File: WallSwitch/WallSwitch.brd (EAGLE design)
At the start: 72 x 54 mm, 37 parts, among them IC1 WS2811, IC2 AT42QT1010-TSHR, IC3 LNK306DG, IC4 WS2811, IC5 AT42QT1010-TSHR, IC6 AP2112K-3.3TRG1, J1 AC Line, J2 Interface

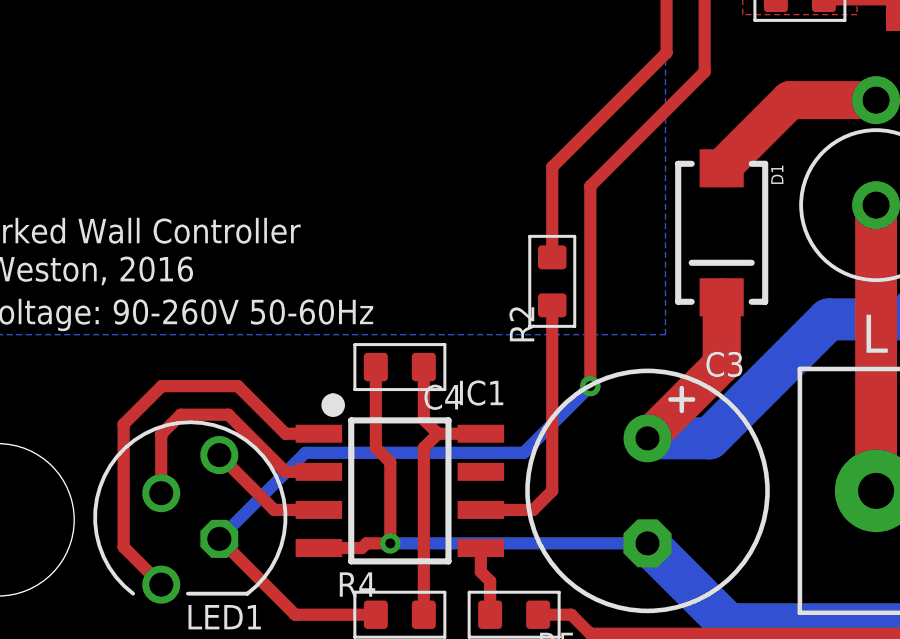
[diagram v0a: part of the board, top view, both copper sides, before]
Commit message: foo
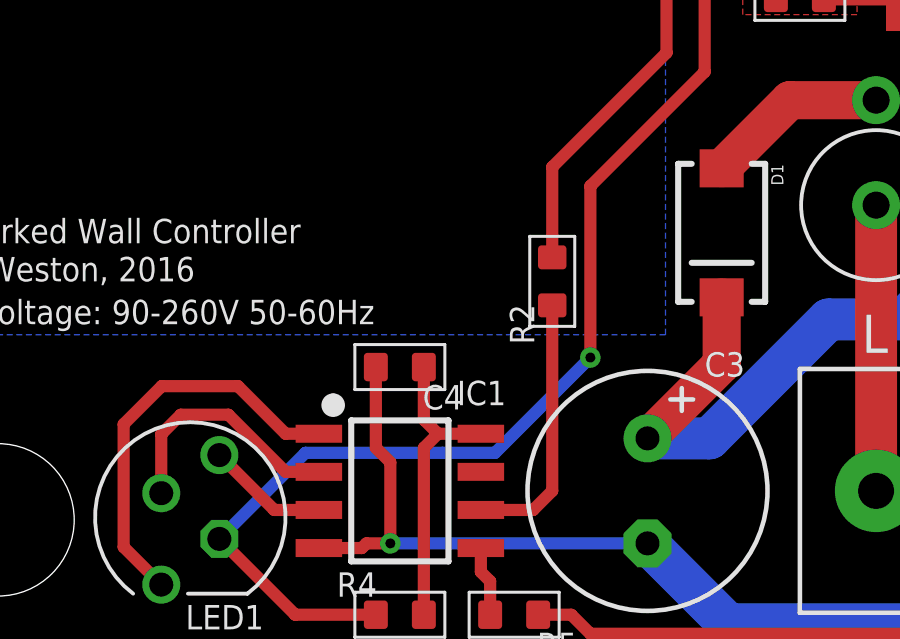
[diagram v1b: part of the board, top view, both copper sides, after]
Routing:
- net +4V: track 117.1 -> 116.5 mm
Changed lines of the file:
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@@
 <layer number="17" name="Pads" color="2" fill="1" visible="yes" active="yes"/>
 <layer number="18" name="Vias" color="2" fill="1" visible="yes" active="yes"/>
-<layer number="19" name="Unrouted" color="6" fill="1" visible="no" active="yes"/>
+<layer number="19" name="Unrouted" color="6" fill="1" visible="yes" active="yes"/>
 <layer number="20" name="Dimension" color="15" fill="1" visible="yes" active="yes"/>
 <layer number="21" name="tPlace" color="7" fill="1" visible="yes" active="yes"/>
@@
 <wire x1="40.005" y1="33.02" x2="38.06" y2="33.02" width="1.016" layer="1"/>
 <wire x1="42.545" y1="34.9975" x2="42.545" y2="32.115" width="1.016" layer="1"/>
-<wire x1="21.2725" y1="6.985" x2="23.495" y2="9.2075" width="0.4064" layer="16"/>
-<via x="23.495" y="9.2075" extent="1-16" drill="0.3302"/>
-<wire x1="23.495" y1="9.2075" x2="23.495" y2="15.875" width="0.4064" layer="1"/>
+<via x="23.495" y="10.16" extent="1-16" drill="0.3302"/>
+<wire x1="23.495" y1="10.16" x2="23.495" y2="15.875" width="0.4064" layer="1"/>
 <wire x1="23.495" y1="15.875" x2="27.305" y2="19.685" width="0.4064" layer="1"/>
 <wire x1="27.305" y1="19.685" x2="27.305" y2="30.48" width="0.4064" layer="1"/>
@@
 <wire x1="36.51" y1="38.0699" x2="37.1174" y2="38.0699" width="0.4064" layer="1"/>
 <wire x1="38.1" y1="33.06" x2="38.06" y2="33.02" width="0.254" layer="1"/>
-<wire x1="21.2725" y1="6.985" x2="13.9984" y2="6.985" width="0.4064" layer="16"/>
+<wire x1="18.57375" y1="6.985" x2="13.9984" y2="6.985" width="0.4064" layer="16"/>
 <wire x1="13.9984" y1="6.985" x2="11.1284" y2="4.115" width="0.4064" layer="16"/>
 <wire x1="16.345" y1="1.5875" x2="13.6559" y2="1.5875" width="0.4064" layer="1"/>
@@
 <wire x1="31.75" y1="34.925" x2="27.305" y2="30.48" width="0.4064" layer="1"/>
 <wire x1="34.61" y1="34.925" x2="36.155" y2="34.925" width="0.4064" layer="1"/>
+<wire x1="18.57375" y1="6.985" x2="20.32" y2="6.985" width="0.4064" layer="16"/>
+<wire x1="20.32" y1="6.985" x2="23.495" y2="10.16" width="0.4064" layer="16"/>
 </signal>
 <signal name="+3.3V">
